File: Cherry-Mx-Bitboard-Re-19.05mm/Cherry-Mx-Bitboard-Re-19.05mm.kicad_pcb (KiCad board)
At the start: 2 copper layers, 17.8 x 17.8 mm, 11 parts, among them SW1 SW_Push

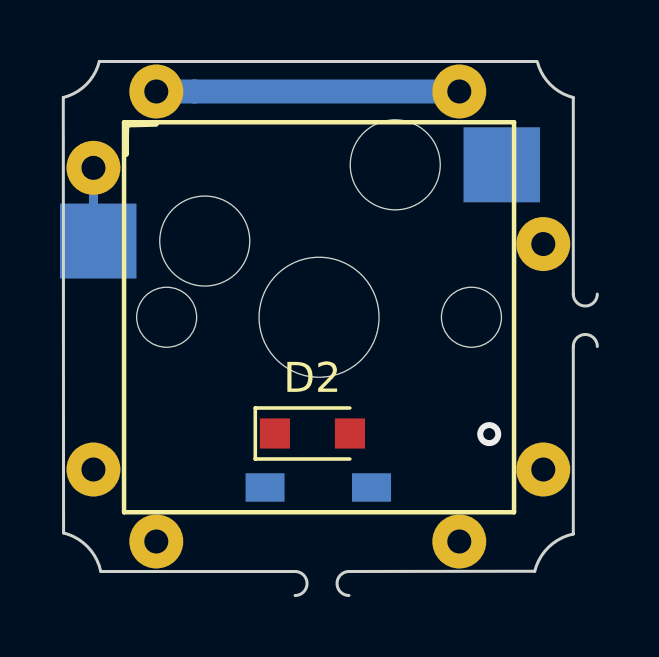
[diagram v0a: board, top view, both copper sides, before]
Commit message: connect everything
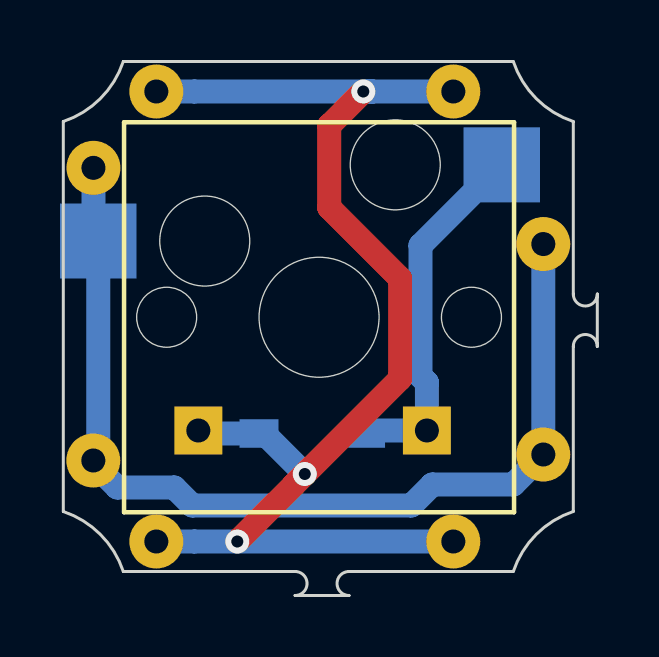
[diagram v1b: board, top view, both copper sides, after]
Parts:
- D2: footprint Diode_SMD:D_SOD-323_HandSoldering -> Footprints:1N4148W; moved to B.Cu
- moved D1 4.43 mm to (88.6, 57.6)
- moved Row114 0.50 mm to (100.1, 58.4)
- moved Row112 0.30 mm to (85.1, 58.6)
- moved Col112 0.20 mm to (97.1, 46.3)
- moved Col114 0.20 mm to (97.1, 61.3)
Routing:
- net Col1: track 10.1 -> 43.3 mm, vias 1 -> 3
- net Row1: track 3.02 -> 34.9 mm
- net Net-(D1-Pad2): track 0.03 -> 12.2 mm
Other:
- outline, holes or cut-outs redrawn
- board text added: "Protocases.com"
- board text added: "v1.1"
